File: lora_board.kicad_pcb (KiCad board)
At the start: 2 copper layers, 20 x 45 mm, 32 parts, among them J1 USB_C_Receptacle_USB2.0_16P, J2 Conn_01x02_Shielded, J3 Conn_01x05, J4 Conn_01x02, Q1 AO3400A, SW1 SW_Push, SW2 SW_SPDT, U1 E73-2G4M08S1C, U2 AP2112K-3.3, U3 E22-900MM22S, U4 MCP73831-2-OT

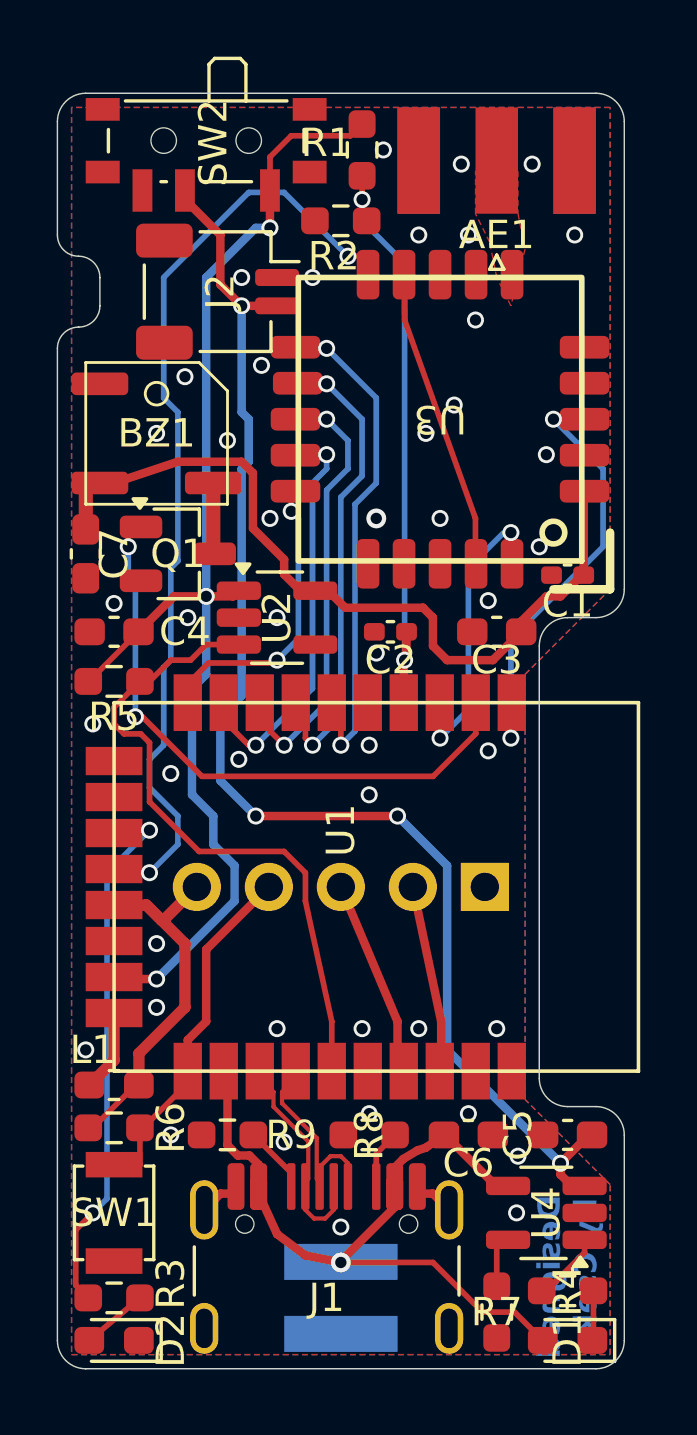
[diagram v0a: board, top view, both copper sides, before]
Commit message: v2 rc2
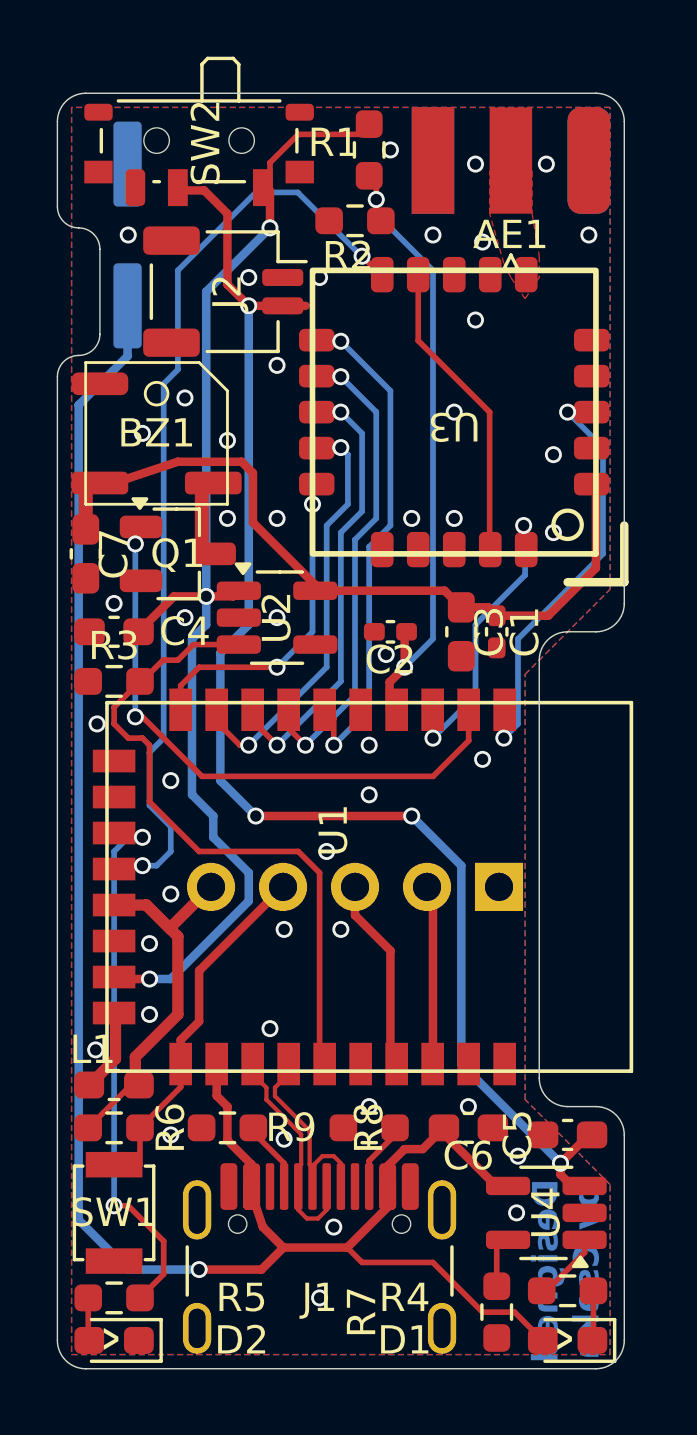
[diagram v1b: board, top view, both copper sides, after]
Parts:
- J4: value Conn_01x02 -> Qi Charger; footprint Library:1x02 smd 2.54 -> Library:QiCharger
- R3: renamed from R5; value 10k -> 1M
- R4: value 1k -> 330
- R5: renamed from R3; value 1k -> 330
- R6: value 10k -> 5.1k
- U3: footprint Library:E22-900MM22S_handsolder -> Library:E22-900MM22S
- moved J4 37.5 mm to (105.5, 80.0)
- moved C1 3.20 mm to (110.5, 94.0), turned to -90 degrees
- moved C3 1.25 mm to (109.2, 94.0), turned to -90 degrees
- moved U3 0.56 mm to (109.0, 86.2)
- moved AE1 0.50 mm to (111.0, 77.5)
- moved J3 0.50 mm to (110.6, 103.0)
- moved R2 0.50 mm to (105.5, 79.5)
- moved C6 0.25 mm to (109.5, 111.5)
- moved J1 0.25 mm to (104.2, 117.5)
- moved J2 0.25 mm to (101.0, 82.0)
- moved R1 0.25 mm to (106.0, 77.0)
- moved R8 0.25 mm to (106.0, 111.5)
- moved R9 0.25 mm to (101.0, 111.5)
- moved SW2 0.25 mm to (100.0, 77.0)
- moved U1 0.25 mm to (105.8, 103.0)
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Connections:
- R3 pad 1: /REG_EN -> GND
- R3 pad 2: VCC -> /REG_EN
- U3 pad 17: unconnected-(U3-NC-Pad17) -> GND
- U3 pad 4: unconnected-(U3-NC-Pad4) -> GND
- U3 pad 5: unconnected-(U3-NC-Pad5) -> GND
- U3 pad 8: unconnected-(U3-NC-Pad8) -> GND
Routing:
- net +5V: track 26.8 -> 68.3 mm
- net GND: track 2.72 -> 0.00 mm, vias 45 -> 46
- net +3.3V: track 28.9 -> 26.9 mm
- net VCC: track 44.1 -> 42.1 mm
- net +BATT: track 47.3 -> 49.2 mm
- net /BAT_SENSE: track 21.1 -> 22.9 mm
- net /BUZZER: track 21.9 -> 21.0 mm
- net Net-(D2-A): track 2.33 -> 1.52 mm
- net Net-(BZ1--): track 2.52 -> 3.26 mm
- net /SCK: track 10.8 -> 11.6 mm
- net VDD: track 13.6 -> 14.3 mm
- net /RXEN: track 33.5 -> 33.0 mm
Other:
- outline, holes or cut-outs redrawn
- board text added: ">"
- board text added: "LSBN v2"
- board text added: "SWCLK"
- board text added: "SWIO"
- board text added: "VREF"
- board text removed: "+"
- board text removed: "-"
- board text removed: "3V3"
- board text removed: "LORA Small v2"
- board text removed: "SWC"
- board text removed: "SWI"
